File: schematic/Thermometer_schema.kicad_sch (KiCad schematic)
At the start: 14 parts, among them J1 USB C, SW1 SW_Push, U1 ESP-12F, U2 SHT21, U3 SSD1306

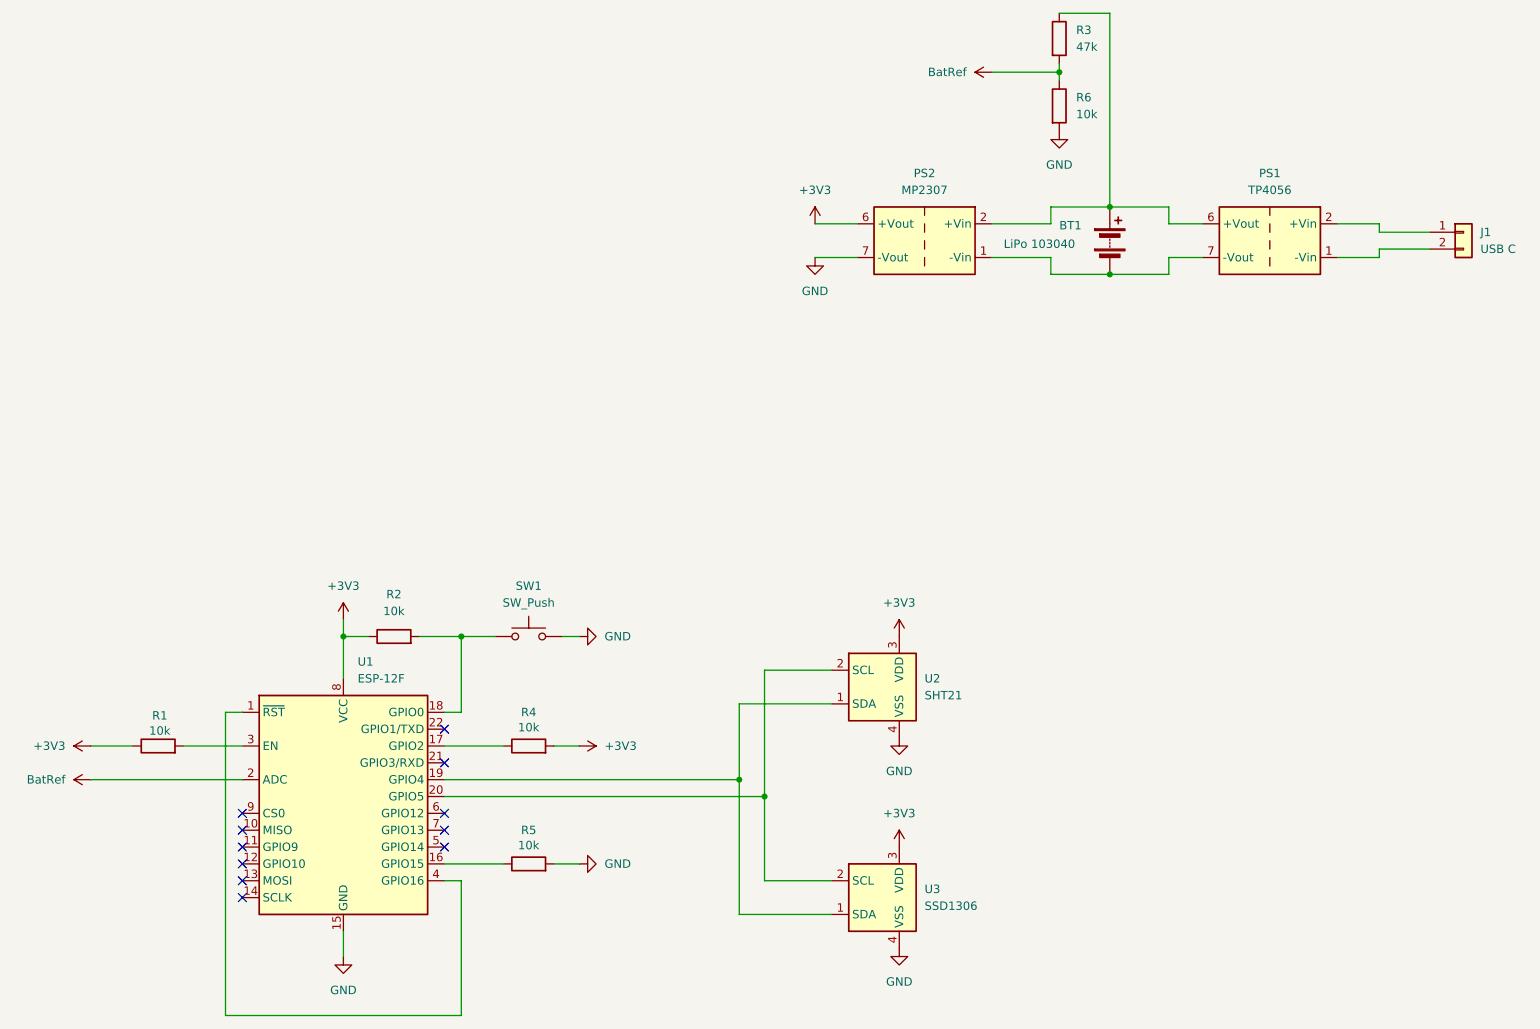
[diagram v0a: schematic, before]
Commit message: Sleep mode (faulty)
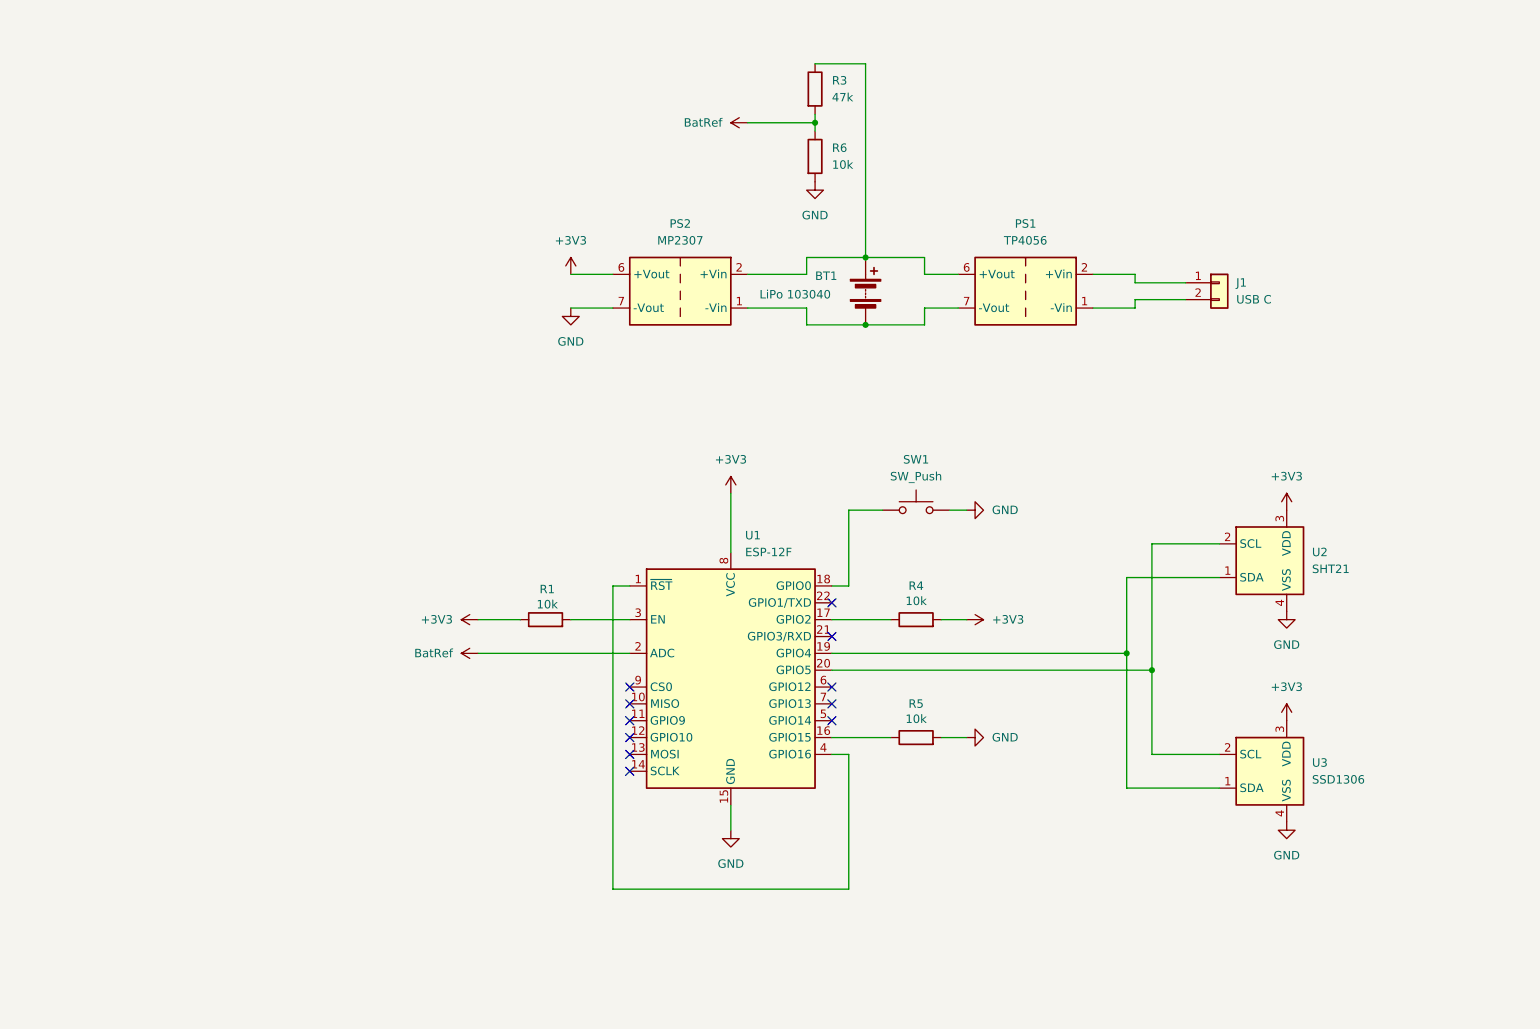
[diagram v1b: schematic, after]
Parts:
- removed R2: 10k, symbol Device:R
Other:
- moved on the sheet: BT1, J1, PS1, PS2, R1, R3, R4, R5, R6, SW1, U1, U2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
